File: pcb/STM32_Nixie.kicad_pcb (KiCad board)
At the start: 4 copper layers, 184 parts, among them J1 CON_SAMTEC_14P_2R_1m27_P_KEY_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, J2 CONN_USBC_RCPT_USB2.0_USB4085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, Q1 NFET_250V_10A_TPH1110FNH,L1Q, Q2 NFET_60V_0A5_2N7002KT1G, SW1 ENC_SPST_24PPR_PEC12R-4225F-S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, U1 IC_SR_MC_HV5622PG-G, U2 IC_SR_MC_HV5622PG-G, U3 IC_MCU_STM32F100C4T6B_48LQFP, U4 IC_LVL_ONSEMI_MC14504BDTR2G, U5 REG_SW_BOOST_TI_TLV61046ADBV, U6 REG_SW_BOOST_TI_LM51561HPWPR, U7 REG_LDO_3V3_250mA_TI_LP5907MF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, U8 IC_FTDI_FT231XS, U9 IC_LSW_TI_TPS2552D, X1 XTAL_8M_20PPM_18pF_ECS-80-18-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, X2 XTAL_32K768_10PPM_7pF_ECS-.32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

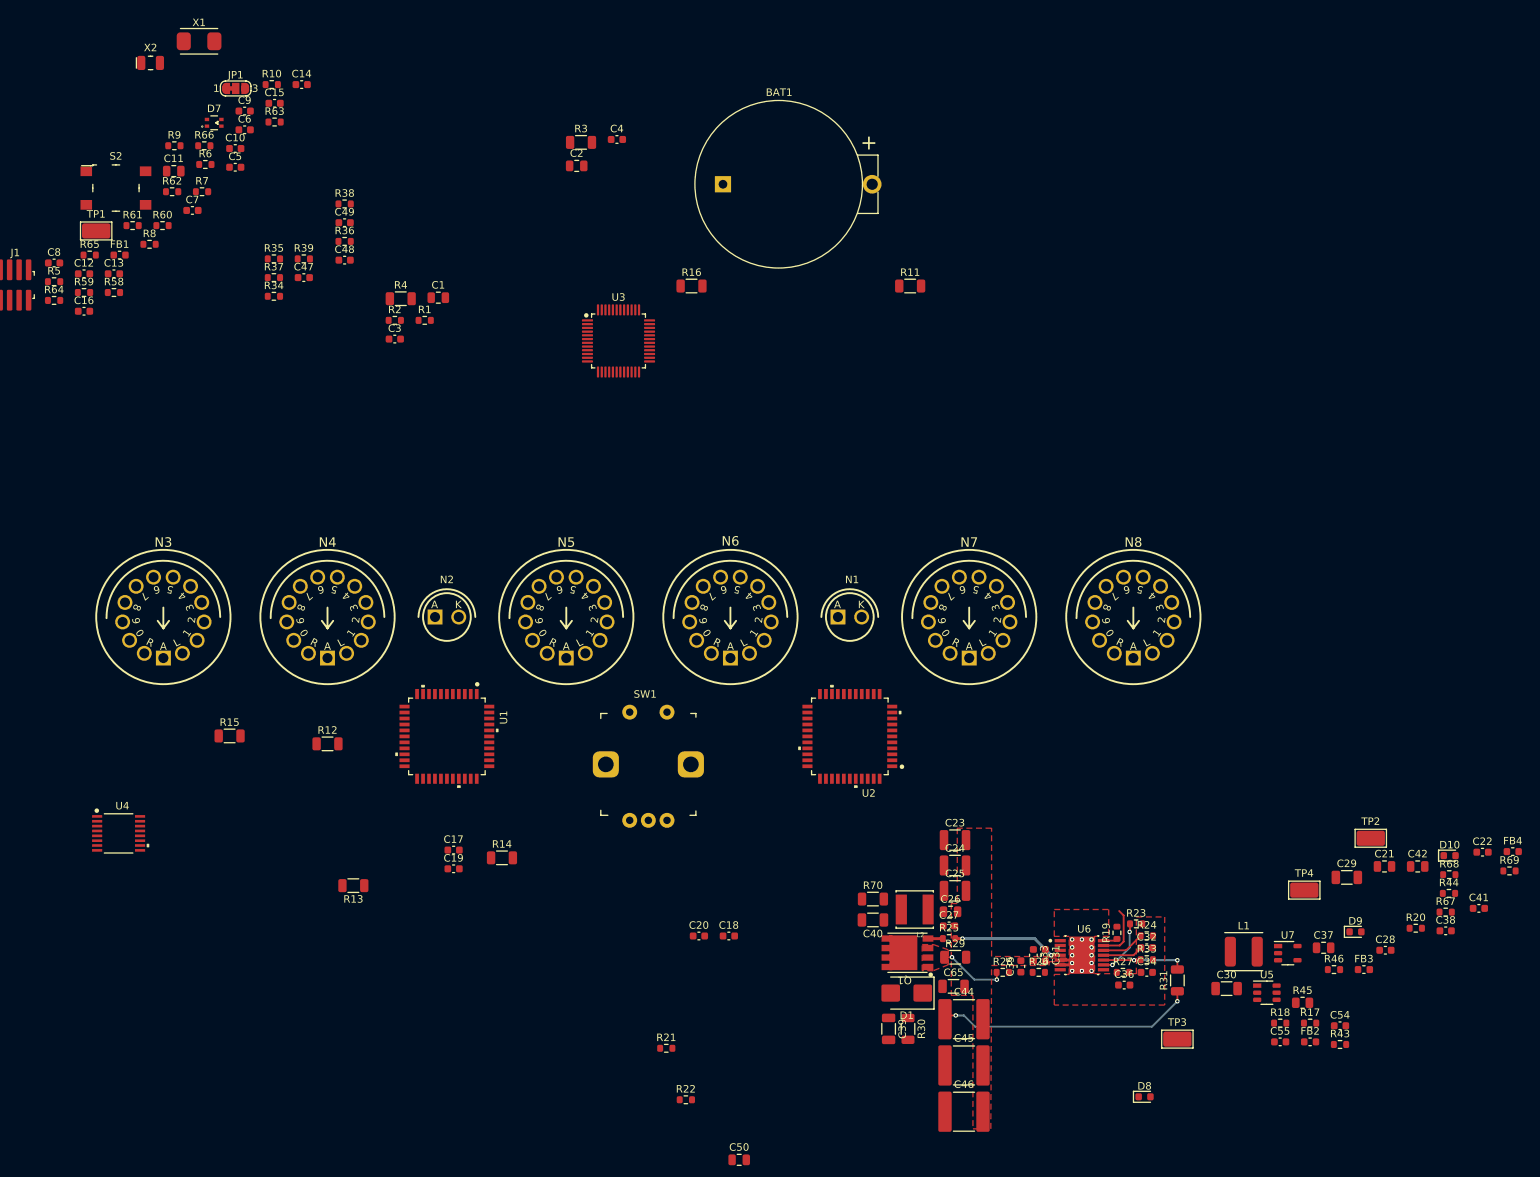
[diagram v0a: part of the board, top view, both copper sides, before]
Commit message: Started mcu placement
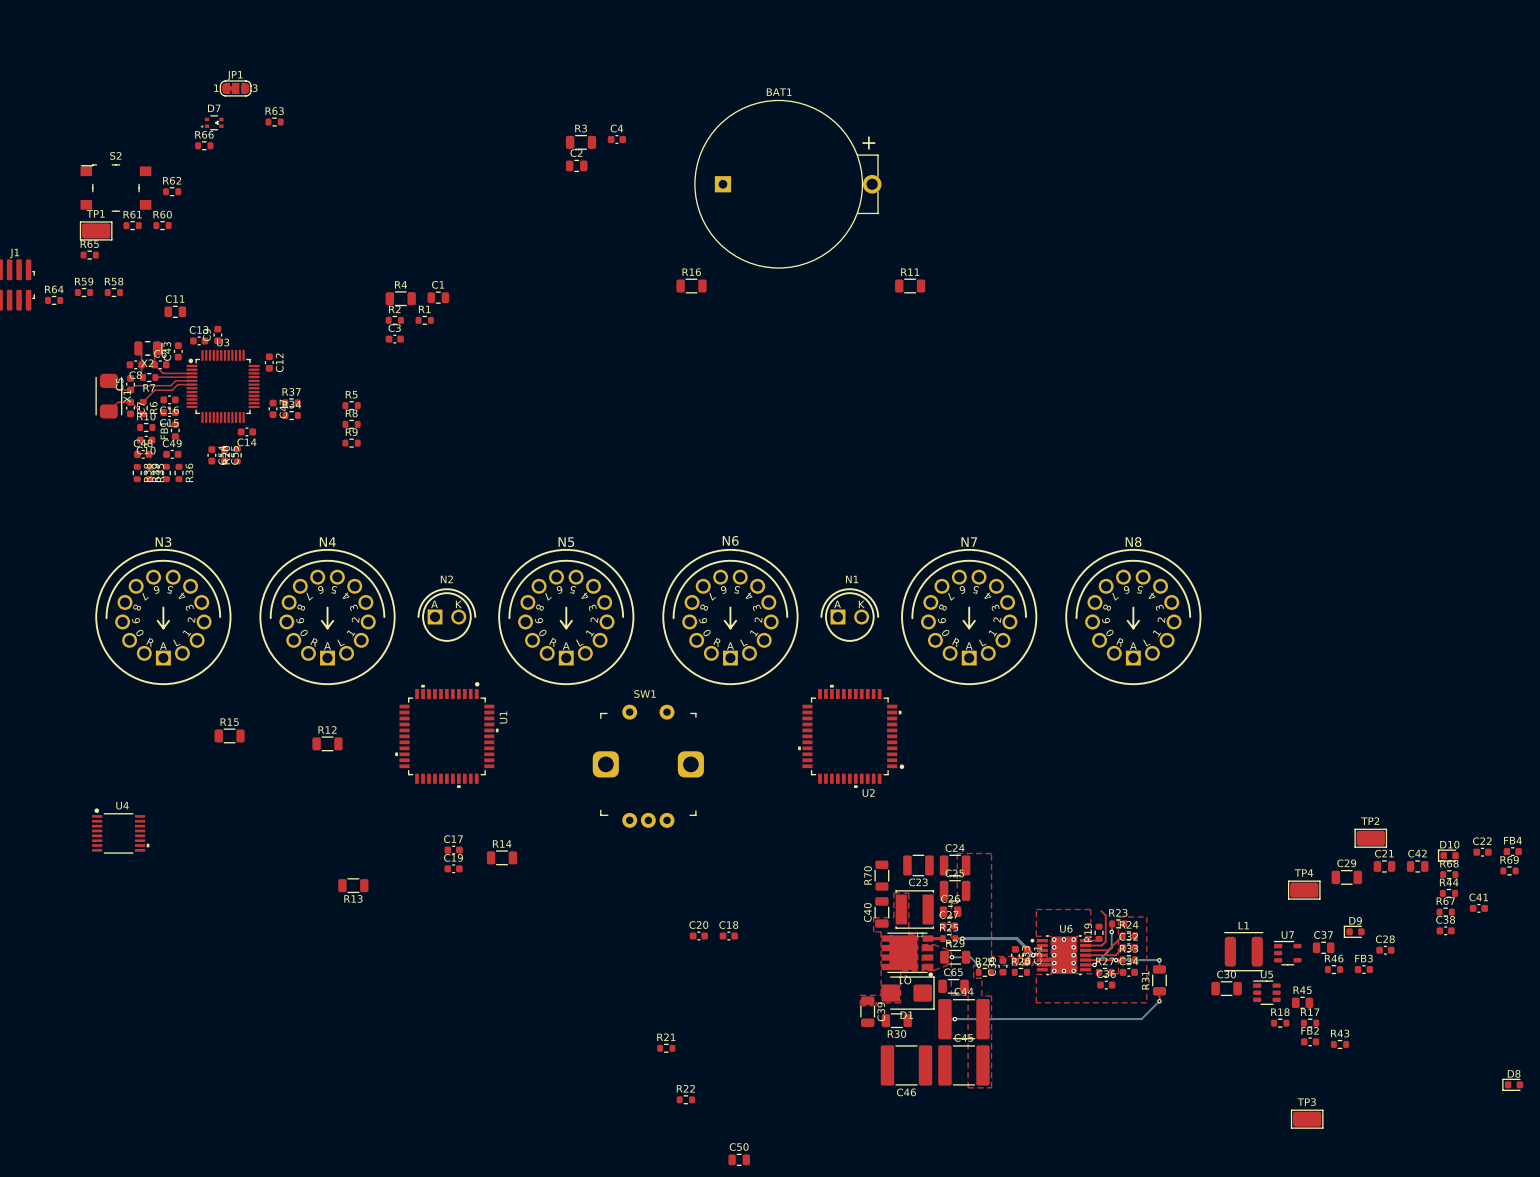
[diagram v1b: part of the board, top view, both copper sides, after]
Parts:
- added C43: CAP_CER_0u1_50V_X7R_0603, Capacitor_SMD:C_0603_1608Metric, F.Cu at (89.0, 51.4)
- moved R20 170.2 mm to (96.9, 65.3), turned to 90 degrees
- moved C54 169.4 mm to (93.5, 65.3), turned to -90 degrees
- moved C55 161.9 mm to (95.2, 65.3), turned to -90 degrees
- moved U3 53.3 mm to (95.0, 56.1)
- moved D8 49.5 mm to (268.0, 149.7)
- moved X1 49.1 mm to (79.7, 57.4), turned to -90 degrees
- moved R10 48.9 mm to (84.7, 61.6)
- moved C14 47.1 mm to (98.2, 62.2), turned to 180 degrees
- moved R9 46.4 mm to (112.2, 63.7)
- moved R38 45.5 mm to (83.5, 67.7), turned to -90 degrees
- moved C15 43.8 mm to (87.8, 59.6), turned to 180 degrees
- moved R5 43.2 mm to (112.2, 58.7)
- moved C10 40.9 mm to (84.7, 63.3), turned to 180 degrees
- moved C49 38.7 mm to (88.2, 65.2)
- moved X2 38.3 mm to (84.9, 51.0), turned to 180 degrees
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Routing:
- net /MCU/OSC_IN: track 0.00 -> 12.2 mm
- net /MCU/OSC32_IN: track 0.00 -> 7.82 mm
- net /MCU/OSC_OUT: track 0.00 -> 7.50 mm
- net /MCU/OSC_OUT_R: track 0.00 -> 5.77 mm
- net /MCU/OSC32_OUT: track 0.00 -> 4.93 mm
- net /MCU/OSC32_OUT_R: track 0.00 -> 4.16 mm
- net /Power/CS_RAW: track 9.27 -> 6.01 mm
- net 180V: track 34.8 -> 31.5 mm
- net /Power/GATE_R: track 15.0 -> 12.6 mm
- added copper zone on F.Cu, net /Power/SW_180V
